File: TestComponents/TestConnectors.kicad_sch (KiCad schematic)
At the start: 11 parts, among them J2-1 Conn_01x04_Male, J2-2 Conn_01x04_Male

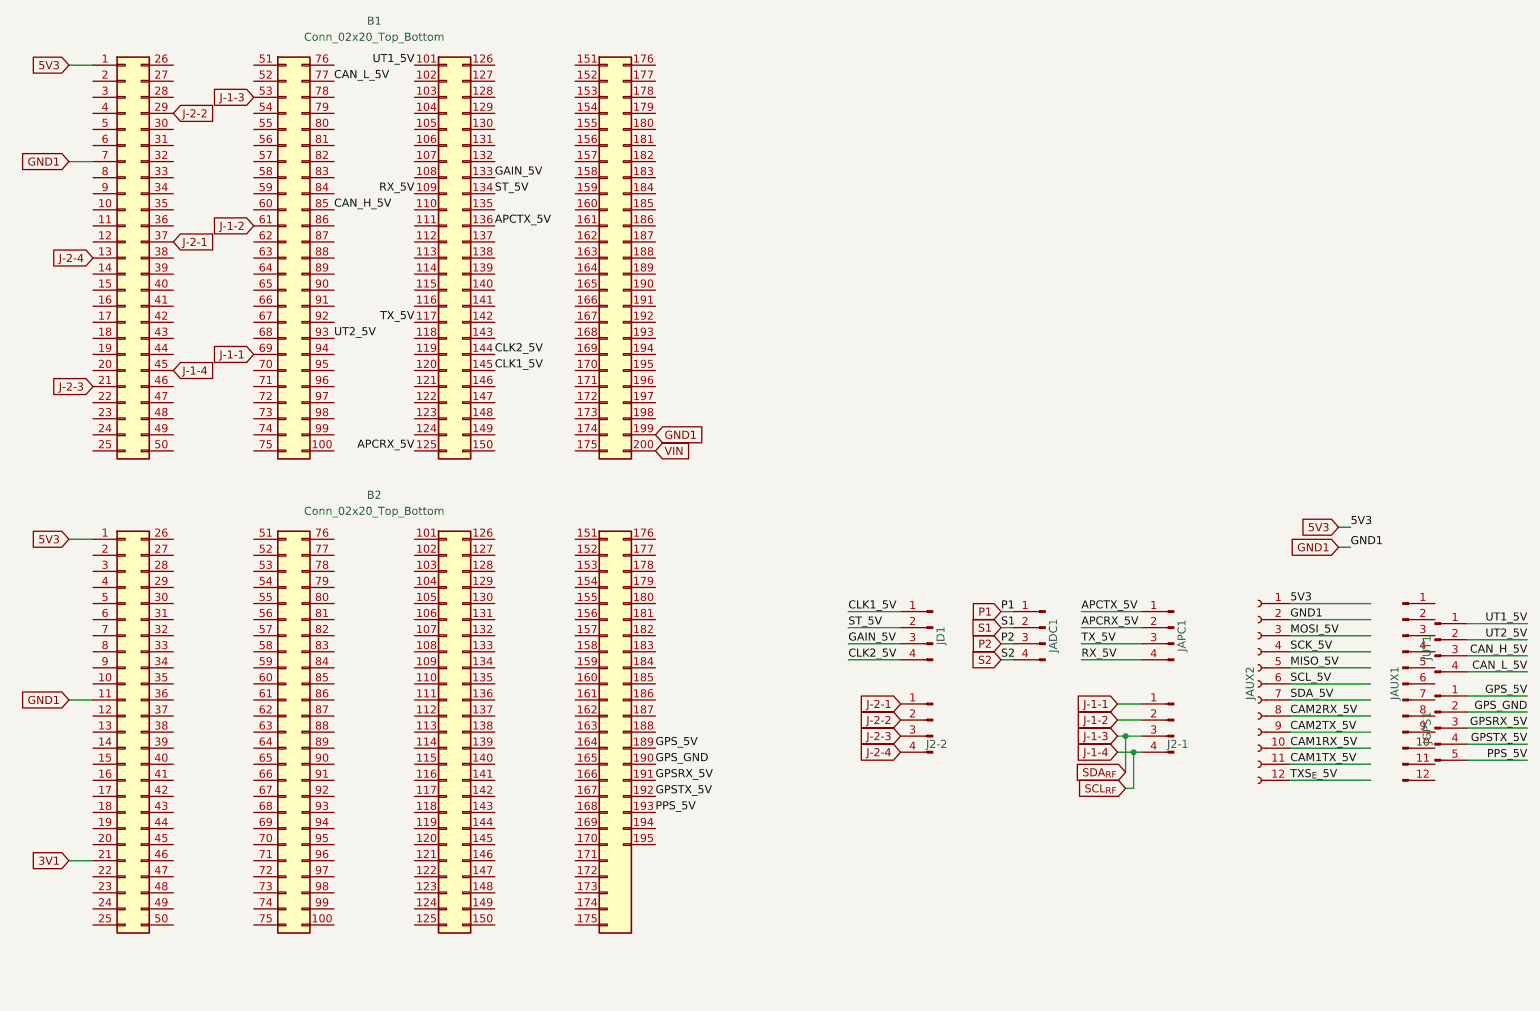
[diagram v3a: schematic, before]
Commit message: SpectDrone Development
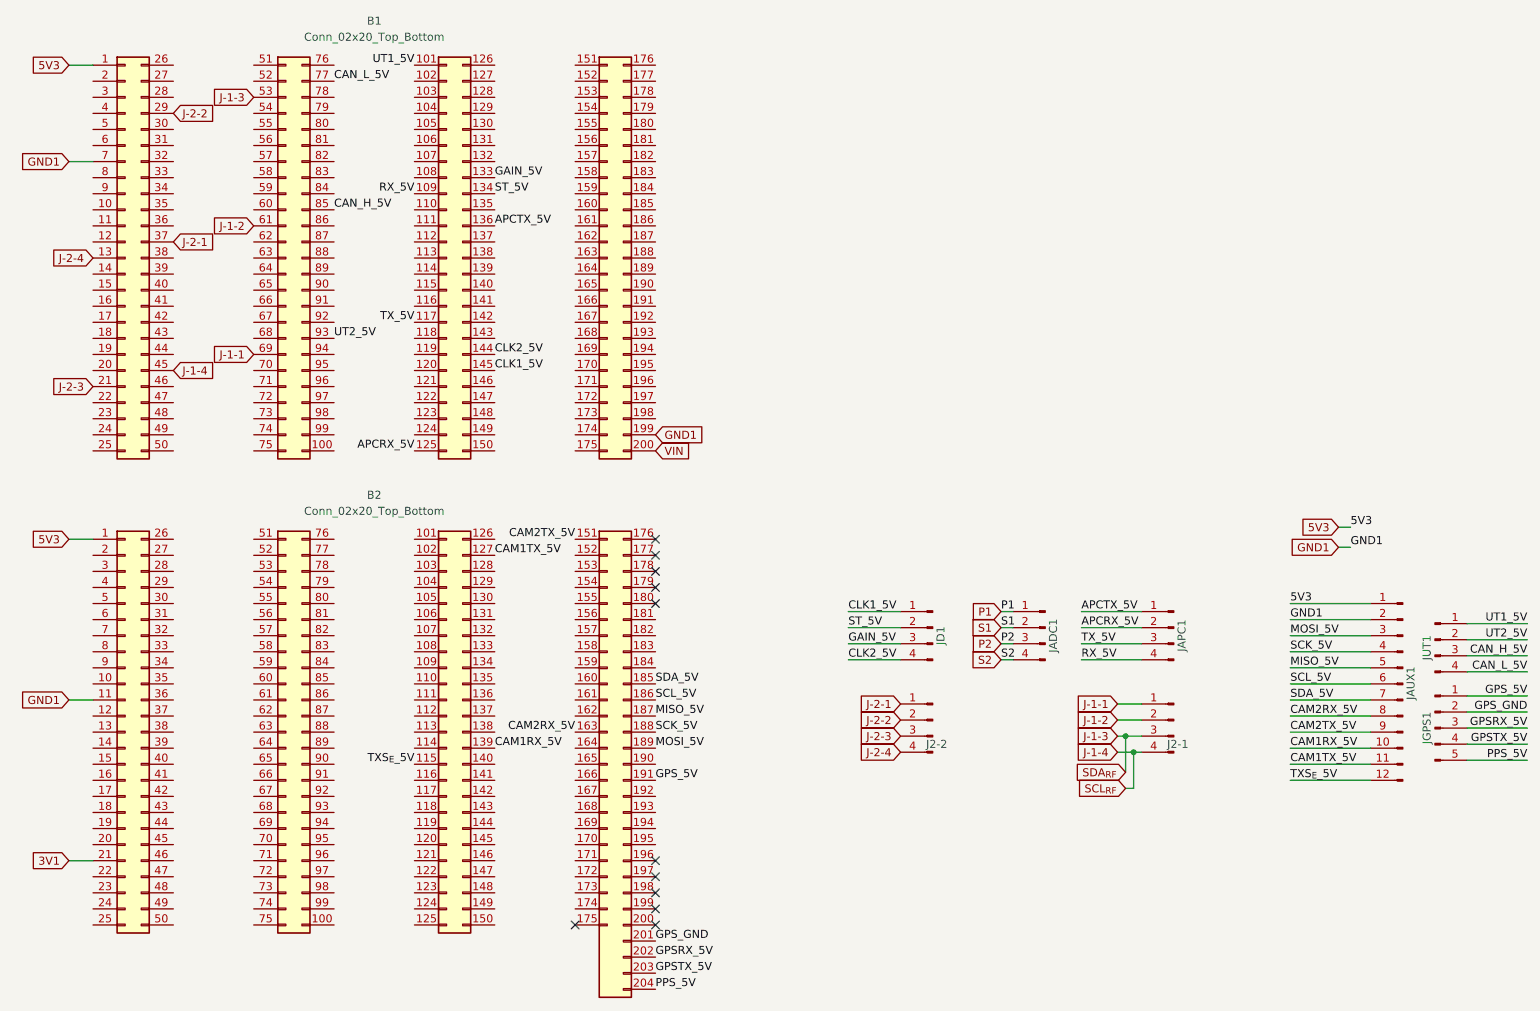
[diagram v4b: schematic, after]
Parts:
- removed JAUX2: AUX, Connector_PinSocket_2.54mm:PinSocket_1x12_P2.54mm_Vertical, symbol Connector:Conn_01x12_Female
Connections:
- net 5V3: now also JAUX1.1 (Pin_1)
- net CAM1RX_5V: now also B2.139 (Pin_139), JAUX1.10 (Pin_10)
- net CAM1TX_5V: now also B2.127 (Pin_127), JAUX1.11 (Pin_11)
- net CAM2RX_5V: now also B2.163 (Pin_163), JAUX1.8 (Pin_8)
- net CAM2TX_5V: now also B2.151 (Pin_151), JAUX1.9 (Pin_9)
- net GND1: now also JAUX1.2 (Pin_2)
- net GPSRX_5V: now also B2.202 (Pin_202); no longer B2.191 (Pin_191)
- net GPSTX_5V: now also B2.203 (Pin_203); no longer B2.192 (Pin_192)
- net GPS_5V: now also B2.191 (Pin_191); no longer B2.189 (Pin_189)
- net GPS_GND: now also B2.201 (Pin_201); no longer B2.190 (Pin_190)
- net MISO_5V: now also B2.187 (Pin_187), JAUX1.5 (Pin_5)
- net MOSI_5V: now also B2.189 (Pin_189), JAUX1.3 (Pin_3)
- net PPS_5V: now also B2.204 (Pin_204); no longer B2.193 (Pin_193)
- net SCK_5V: now also B2.188 (Pin_188), JAUX1.4 (Pin_4)
- net SCL_5V: now also B2.186 (Pin_186), JAUX1.6 (Pin_6)
- net SDA_5V: now also B2.185 (Pin_185), JAUX1.7 (Pin_7)
- net TXS_{E}_5V: now also B2.115 (Pin_115), JAUX1.12 (Pin_12)
- no-connect marks 0 -> 11
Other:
- moved on the sheet: JAUX1
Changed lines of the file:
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@@
   (junction (at 205.74 146.685) (diameter 0) (color 0 0 0 0)
   )
+  (no_connect (at 130.175 168.91))
+  (no_connect (at 130.175 171.45))
+  (no_connect (at 130.175 173.99))
+  (no_connect (at 117.475 173.99))
+  (no_connect (at 130.175 113.03))
+  (no_connect (at 130.175 115.57))
+  (no_connect (at 130.175 118.11))
+  (no_connect (at 130.175 120.65))
+  (no_connect (at 130.175 123.19))
+  (no_connect (at 130.175 166.37))
+  (no_connect (at 130.175 163.83))
   (wire (pts (xy 184.785 129.54) (xy 186.69 129.54))
     (stroke (width 0) (type default) (color 0 0 0 0))
@@
     (effects (font (size 1.27 1.27)) (justify left bottom))
   )
+  (label "MOSI_5V" (at 130.175 146.05 0)
+    (effects (font (size 1.27 1.27)) (justify left bottom))
+  )
   (label "GND1" (at 240.03 114.3 0)
     (effects (font (size 1.27 1.27)) (justify left bottom))
@@
     (effects (font (size 1.27 1.27)) (justify left bottom))
   )
+  (label "CAM1TX_5V" (at 104.775 115.57 0)
+    (effects (font (size 1.27 1.27)) (justify left bottom))
+  )
   (label "MOSI_5V" (at 230.505 128.27 0)
     (effects (font (size 1.27 1.27)) (justify left bottom))
@@
     (effects (font (size 1.27 1.27)) (justify right bottom))
   )
+  (label "MISO_5V" (at 130.175 140.97 0)
+    (effects (font (size 1.27 1.27)) (justify left bottom))
+  )
   (label "RX_5V" (at 197.485 132.08 0)
     (effects (font (size 1.27 1.27)) (justify left bottom))
@@
     (effects (font (size 1.27 1.27)) (justify left bottom))
   )
-  (label "GPSRX_5V" (at 130.175 151.13 0)
-    (effects (font (size 1.27 1.27)) (justify left bottom))
-  )
-  (label "PPS_5V" (at 130.175 156.21 0)
+  (label "GPSRX_5V" (at 130.175 179.07 0)
+    (effects (font (size 1.27 1.27)) (justify left bottom))
+  )
+  (label "PPS_5V" (at 130.175 184.15 0)
     (effects (font (size 1.27 1.27)) (justify left bottom))
   )
@@
     (effects (font (size 1.27 1.27)) (justify left bottom))
   )
+  (label "TXS_{E}_5V" (at 92.075 148.59 180)
+    (effects (font (size 1.27 1.27)) (justify right bottom))
+  )
+  (label "SCK_5V" (at 130.175 143.51 0)
+    (effects (font (size 1.27 1.27)) (justify left bottom))
+  )
   (label "CAN_H_5V" (at 79.375 60.96 0)
     (effects (font (size 1.27 1.27)) (justify left bottom))
@@
     (effects (font (size 1.27 1.27)) (justify left bottom))
   )
+  (label "CAM2RX_5V" (at 117.475 143.51 180)
+    (effects (font (size 1.27 1.27)) (justify right bottom))
+  )
   (label "S1" (at 184.785 127 0)
     (effects (font (size 1.27 1.27)) (justify left bottom))
   )
+  (label "SCL_5V" (at 130.175 138.43 0)
+    (effects (font (size 1.27 1.27)) (justify left bottom))
+  )
+  (label "CAM1RX_5V" (at 104.775 146.05 0)
+    (effects (font (size 1.27 1.27)) (justify left bottom))
+  )
   (label "ST_5V" (at 104.775 58.42 0)
     (effects (font (size 1.27 1.27)) (justify left bottom))
@@
     (effects (font (size 1.27 1.27)) (justify right bottom))
   )
+  (label "CAM2TX_5V" (at 117.475 113.03 180)
+    (effects (font (size 1.27 1.27)) (justify right bottom))
+  )
   (label "ST_5V" (at 160.655 127 0)
     (effects (font (size 1.27 1.27)) (justify left bottom))
@@
     (effects (font (size 1.27 1.27)) (justify left bottom))
   )
-  (label "GPSTX_5V" (at 130.175 153.67 0)
-    (effects (font (size 1.27 1.27)) (justify left bottom))
-  )
-  (label "GPS_5V" (at 130.175 146.05 0)
-    (effects (font (size 1.27 1.27)) (justify left bottom))
-  )
-  (label "GPS_GND" (at 130.175 148.59 0)
+  (label "GPSTX_5V" (at 130.175 181.61 0)
+    (effects (font (size 1.27 1.27)) (justify left bottom))
+  )
+  (label "GPS_5V" (at 130.175 151.13 0)
+    (effects (font (size 1.27 1.27)) (justify left bottom))
+  )
+  (label "GPS_GND" (at 130.175 176.53 0)
     (effects (font (size 1.27 1.27)) (justify left bottom))
   )
   (label "GPS_GND" (at 267.97 140.335 180)
     (effects (font (size 1.27 1.27)) (justify right bottom))
+  )
+  (label "SDA_5V" (at 130.175 135.89 0)
+    (effects (font (size 1.27 1.27)) (justify left bottom))
   )
   (label "RX_5V" (at 92.075 58.42 180)
@@
     (pin "194")
     (pin "195")
+    (pin "196")
+    (pin "197")
+    (pin "198")
+    (pin "199")
     (pin "2")
     (pin "20")
+    (pin "200")
+    (pin "201")
+    (pin "202")
+    (pin "203")
+    (pin "204")
     (pin "21")
     (pin "22")
@@
     (pin "4")
   )
-  (symbol (lib_id "Connector:Conn_01x12_Male") (at 248.285 135.89 0) (unit 1)
+  (symbol (lib_id "Connector:Conn_01x12_Male") (at 248.285 135.89 0) (mirror y) (unit 1)
     (in_bom yes) (on_board yes)
-    (property "Reference" "JAUX1" (id 0) (at 247.015 138.43 90)
+    (property "Reference" "JAUX1" (id 0) (at 249.555 138.43 90)
       (effects (font (size 1.27 1.27)) (justify left))
     )
-    (property "Value" "AUX" (id 1) (at 245.745 137.16 90)
+    (property "Value" "AUX" (id 1) (at 250.825 137.16 90)
       (effects (font (size 1.27 1.27)) (justify left) hide)
     )
@@
       (effects (font (size 1.27 1.27)) hide)
     )
-    (pin "1")
-    (pin "10")
-    (pin "11")
-    (pin "12")
-    (pin "2")
-    (pin "3")
-    (pin "4")
-    (pin "5")
-    (pin "6")
-    (pin "7")
-    (pin "8")
-    (pin "9")
-  )
-  (symbol (lib_id "Connector:Conn_01x12_Female") (at 225.425 135.89 0) (mirror y) (unit 1)
-    (in_bom yes) (on_board yes)
-    (property "Reference" "JAUX2" (id 0) (at 224.155 138.43 90)
-      (effects (font (size 1.27 1.27)) (justify left))
-    )
-    (property "Value" "AUX" (id 1) (at 227.965 137.16 90)
-      (effects (font (size 1.27 1.27)) (justify left) hide)
-    )
-    (property "Footprint" "Connector_PinSocket_2.54mm:PinSocket_1x12_P2.54mm_Vertical" (id 2) (at 225.425 135.89 0)
-      (effects (font (size 1.27 1.27)) hide)
-    )
-    (property "Datasheet" "~" (id 3) (at 225.425 135.89 0)
-      (effects (font (size 1.27 1.27)) hide)
-    )
